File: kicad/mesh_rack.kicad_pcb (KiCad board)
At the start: 4 copper layers, 200 x 100 mm, 82 parts, among them J1 Input, J10 Conn_01x02, J11 Conn_01x04, J12 Conn_Coaxial_Small, J2 Power Switch, J3 USB_C_Receptacle_USB2.0_14P, J4 Conn_01x02, J5 BOOT, J6 EN, J7 Conn_Coaxial_Small, J8 Conn_02x09_Counter_Clockwise, J9 Conn_01x10, Q1 IRF9540N, Q2 IRF540N, U1 NEO-M8N, U2 ESP32-S3-WROOM-1, U3 XL1509-5.0, U4 XL1509-3.3, U5 TPD2EUSB30, U6 E22-900M30S, U7 INA260

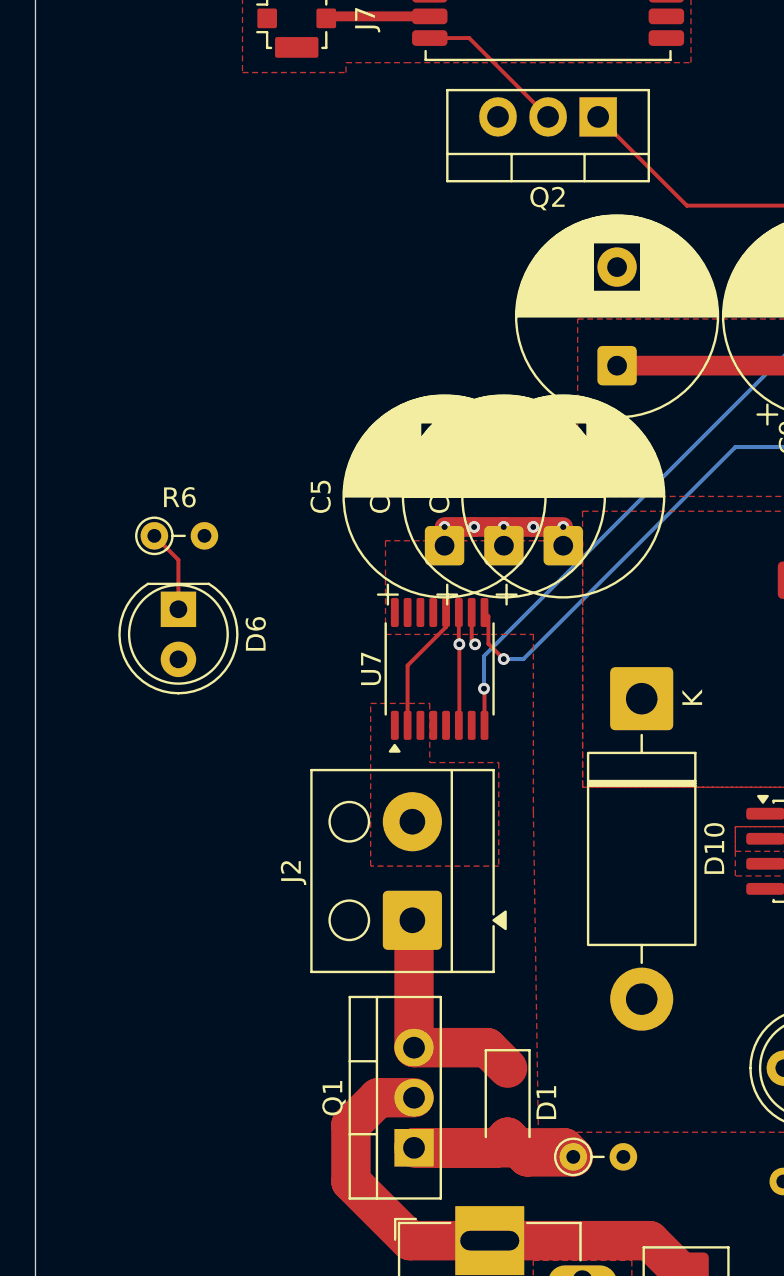
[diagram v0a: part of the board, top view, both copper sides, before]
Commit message: update pcb
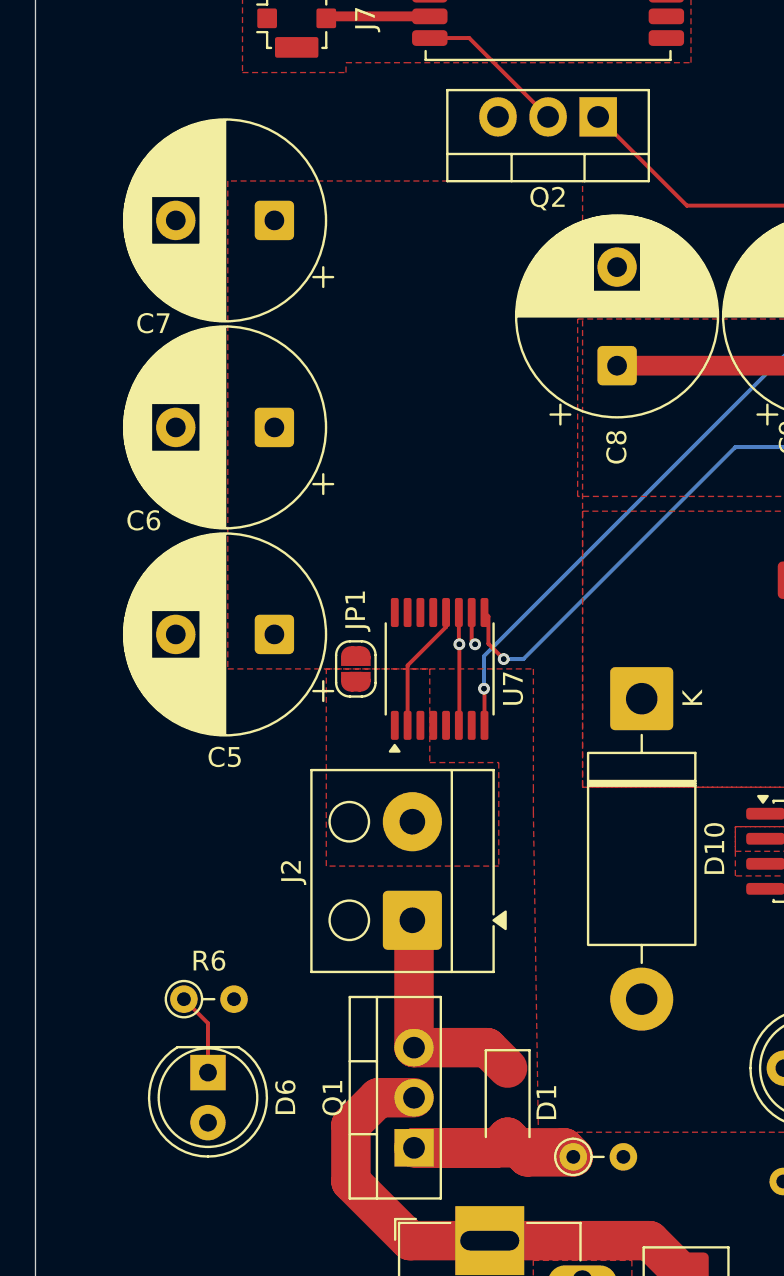
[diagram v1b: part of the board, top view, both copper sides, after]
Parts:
- added JP1: SolderJumper_2_Open, Jumper:SolderJumper-2_P1.3mm_Open_RoundedPad1.0x1.5mm, F.Cu at (41.2, 82.2)
- moved D6 23.5 mm to (33.8, 102.7)
- moved R6 23.5 mm to (32.5, 99.0)
- moved C7 22.1 mm to (37.1, 59.5), turned to 180 degrees
- moved C6 13.1 mm to (37.1, 70.0), turned to 180 degrees
- moved C5 9.73 mm to (37.1, 80.5), turned to 180 degrees
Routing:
- net GND: track 32.6 -> 26.6 mm, vias 34 -> 29
